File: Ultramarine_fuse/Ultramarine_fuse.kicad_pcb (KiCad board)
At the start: 2 copper layers, 152.5 x 126 mm, 142 parts, among them J1 Conn_01x04_Female, J2 Conn_01x04_Female, J3 Conn_01x02_Male, J4 Conn_01x02_Male, Q1 AO3401A, Q2 AO3400A, Q3 AO3400A, SW1 SW_Push, SW10 SW_Push, SW11 SW_Push, SW12 SW_Push, SW13 SW_Push, SW14 SW_Push, SW15 SW_Push, SW16 SW_Push, SW17 SW_Push, SW18 SW_Push, SW19 SW_Push, SW2 SW_Push, SW20 SW_Push, SW21 SW_Push, SW22 SW_Push, SW23 SW_Push, SW24 SW_Push, SW25 SW_Push, SW26 SW_Push, SW27 SW_Push, SW28 SW_Push, SW29 SW_Push, SW3 SW_Push, SW30 SW_Push, SW31 SW_Push, SW32 SW_Push, SW33 SW_Push, SW34 SW_Push, SW35 SW_Push, SW36 SW_Push, SW37 SW_DPDT_x2, SW4 SW_Push, SW5 SW_Push, SW6 SW_Push, SW7 SW_Push, SW8 SW_Push, SW9 SW_Push, U1 Pro_Micro, U10 SK6812mini, U11 SK6812mini, U12 SK6812mini, U13 SK6812mini, U14 SK6812mini, U15 SK6812mini, U16 SK6812mini, U17 SK6812mini, U18 SK6812mini, U19 SK6812mini, U2 SK6812mini, U20 SK6812mini, U21 SK6812mini, U22 SK6812mini, U23 SK6812mini, U24 SK6812mini, U25 SK6812mini, U26 SK6812mini, U27 SK6812mini, U28 SK6812mini, U29 SK6812mini, U3 SK6812mini, U30 SK6812mini, U31 SK6812mini, U32 SK6812mini, U33 SK6812mini, U34 SK6812mini, U35 SK6812mini, U36 SK6812mini, U37 MCP73831, U38 DW01A-G, U4 SK6812mini, U5 SK6812mini, U6 SK6812mini, U7 SK6812mini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

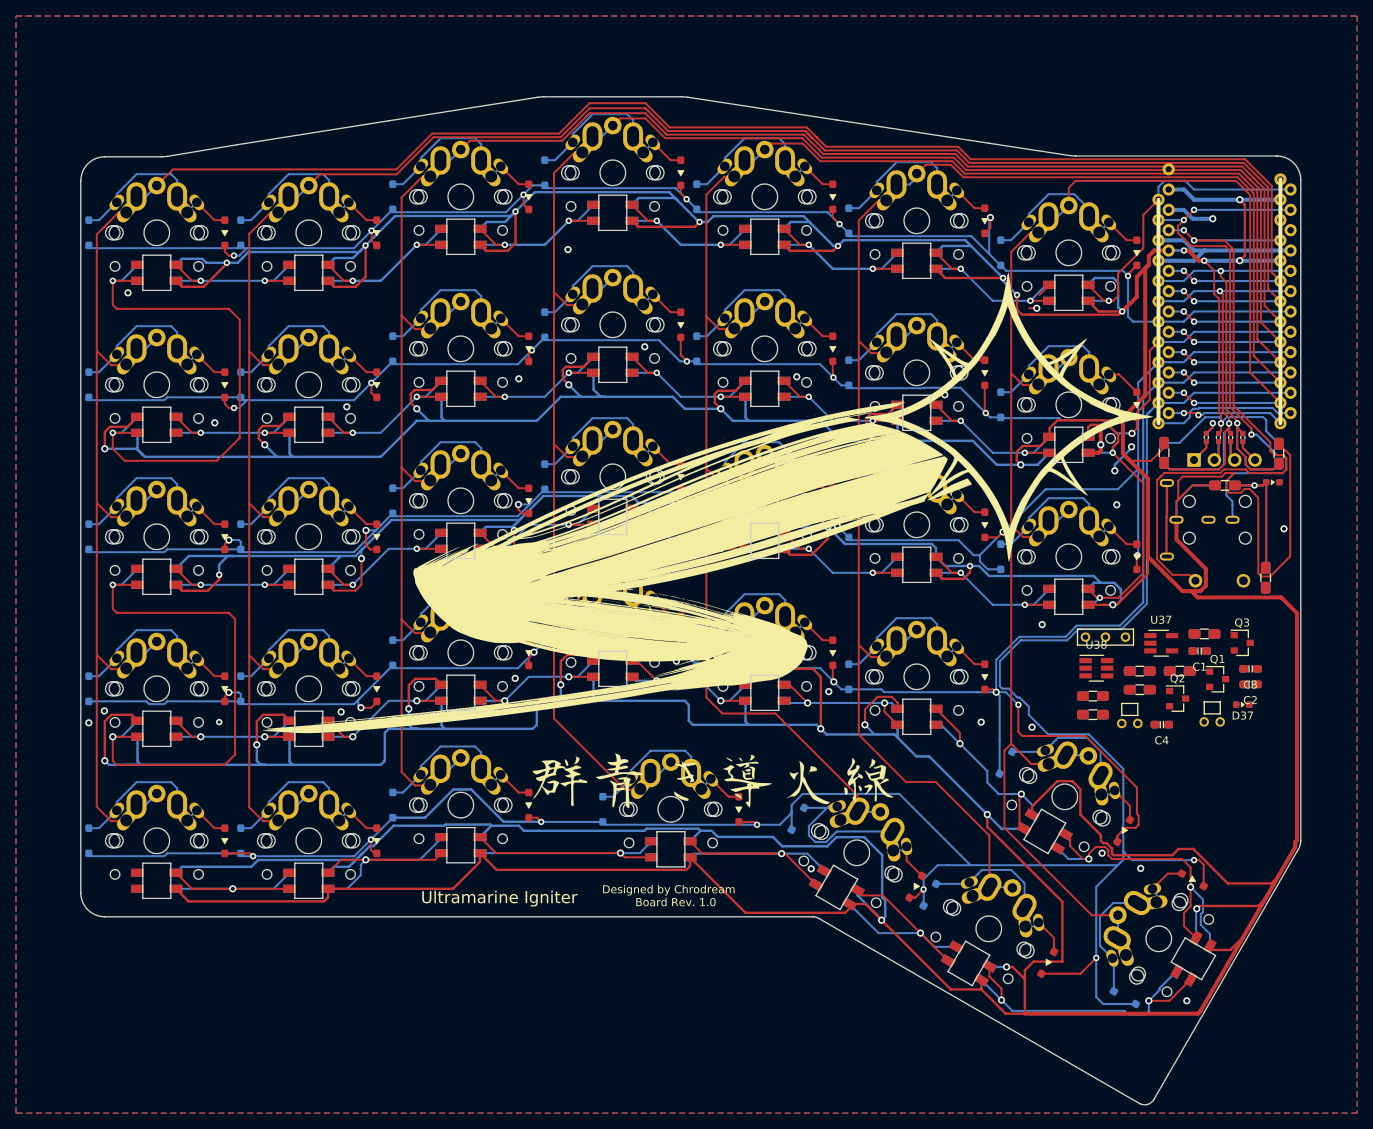
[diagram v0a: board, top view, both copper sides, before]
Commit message: fix circuit
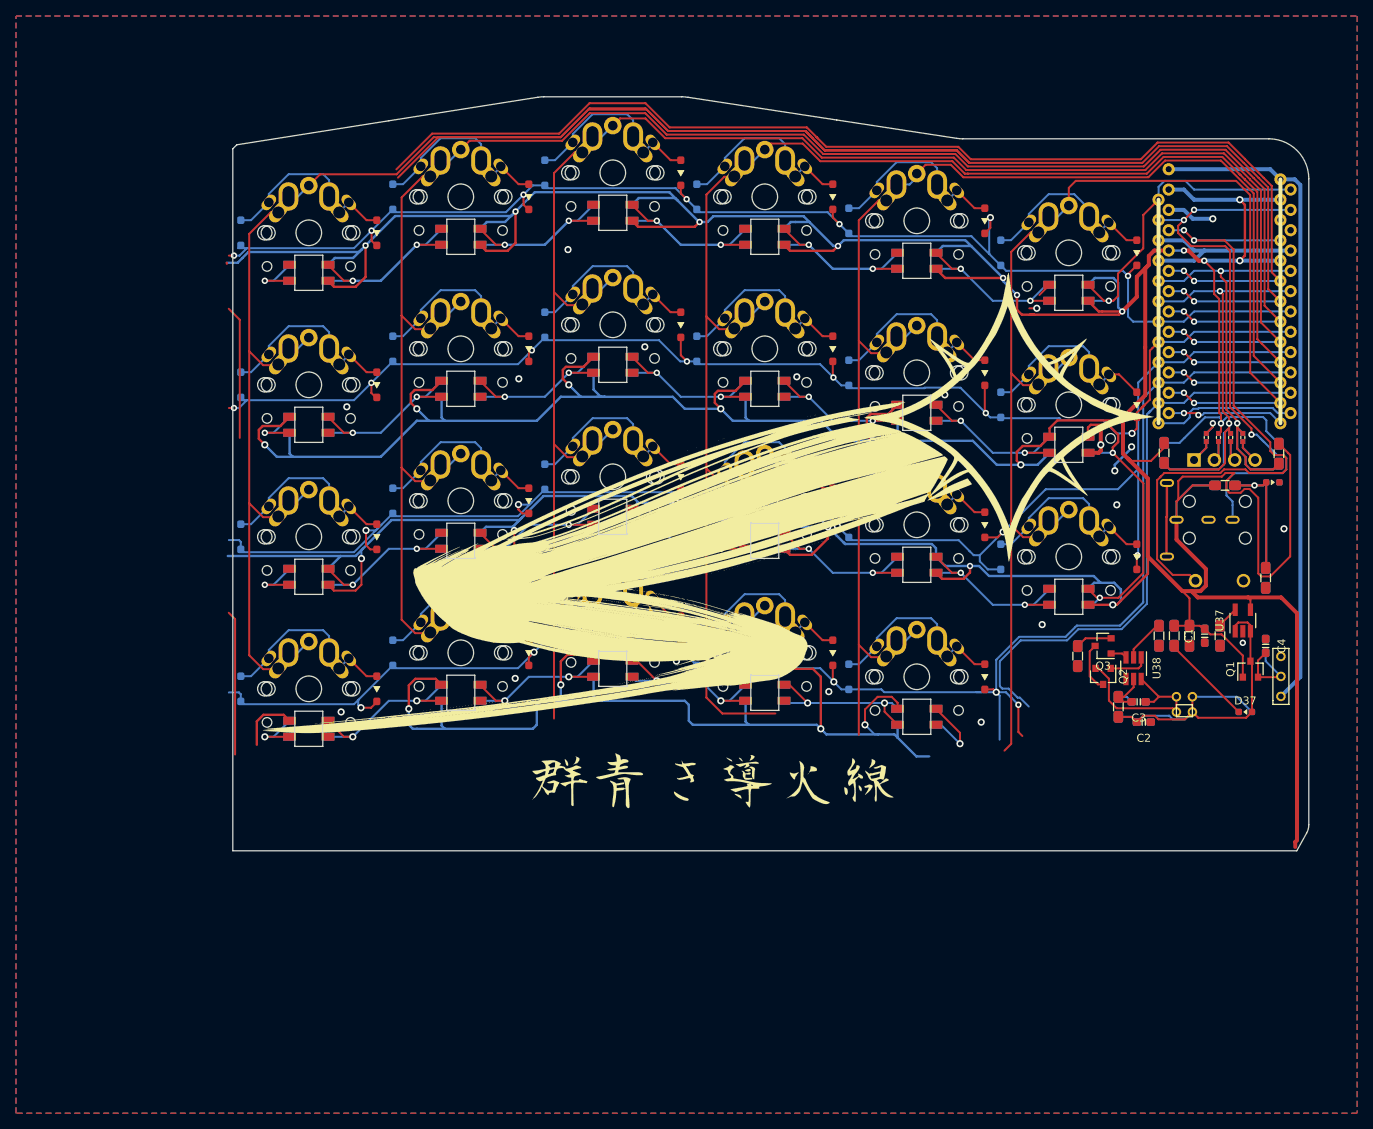
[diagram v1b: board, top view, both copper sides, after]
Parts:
- removed D1, D15, D22, D28, D29, D30, D31, D32, D33, D34, D35, D8: D, Basic_SOP:1N4148
- removed SW1, SW15, SW22, SW28, SW29, SW30, SW31, SW32, SW33, SW34, SW35, SW8: SW_Push, Switch_Keyboard_Cherry_MX:MX-Kailh
- removed U16, U2, U23, U29, U30, U31, U32, U33, U34, U35, U36, U9: SK6812mini, Basic_SOP:SK6812mini
- J4: moved to B.Cu
- moved SW37 22.5 mm to (183.5, 108.0), turned to 90 degrees
- moved R1 17.6 mm to (175.9, 102.9), turned to 90 degrees
- moved Q3 17.4 mm to (161.3, 104.1), turned to 180 degrees
- moved C4 16.3 mm to (181.6, 104.1), turned to 90 degrees
- moved C3 14.6 mm to (165.7, 111.1)
- moved C2 14.2 mm to (166.4, 113.7)
- moved U37 10.6 mm to (178.8, 101.0), turned to 90 degrees
- moved Q2 9.71 mm to (161.3, 108.0), turned to 270 degrees
- moved R6 8.82 mm to (158.1, 105.4), turned to 270 degrees
- moved J4 6.97 mm to (171.4, 112.4)
- moved R2 6.17 mm to (170.2, 102.9), turned to 270 degrees
- moved R7 5.13 mm to (168.3, 102.9), turned to 270 degrees
- moved J3 4.69 mm to (171.4, 110.5), turned to 180 degrees
- moved U38 4.65 mm to (165.1, 106.9), turned to 270 degrees
- moved Q1 4.29 mm to (179.7, 107.0), turned to 90 degrees
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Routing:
- net VCC: track 1503.4 -> 996.6 mm, vias 37 -> 28
- net /Row4: track 309.2 -> 72.2 mm, vias 7 -> 0
- net /Col0: track 297.4 -> 146.0 mm
- net /Bat+: track 0.00 -> 82.2 mm
- net Net-(C2-Pad1): track 0.00 -> 52.9 mm
- net Net-(U2-Pad1): track 68.1 -> 16.7 mm, vias 2 -> 0
- net Net-(U16-Pad1): track 68.8 -> 18.0 mm, vias 2 -> 0
- net /Row3: track 250.2 -> 199.6 mm, vias 7 -> 6
- net /Col6: track 205.1 -> 160.1 mm
- net Net-(U32-Pad3): track 44.6 -> 0.00 mm, vias 1 -> 0
- net Net-(U29-Pad1): track 42.8 -> 0.00 mm, vias 2 -> 0
- net Net-(U35-Pad3): track 40.6 -> 0.00 mm, vias 2 -> 0
- net Net-(U33-Pad3): track 35.9 -> 0.00 mm, vias 1 -> 0
- net /Col1: track 280.9 -> 314.2 mm
- net Net-(U31-Pad3): track 32.9 -> 0.00 mm, vias 1 -> 0
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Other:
- board size 152.5 x 126 mm -> 134.5 x 94.2 mm
- board text removed: "Designed by Chrodream ~ Board Rev. 1.0"
- board text removed: "Ultramarine Igniter"
